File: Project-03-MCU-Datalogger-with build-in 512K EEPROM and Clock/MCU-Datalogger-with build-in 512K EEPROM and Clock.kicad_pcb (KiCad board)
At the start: 2 copper layers, 49.2 x 33.5 mm, 30 parts, among them J1 Conn_01x09_Pin, J2 Conn_01x04_Pin, J4 Conn_02x03_Odd_Even, U1 DS1337S_, U2 24LC1025, U3 24LC1025, U4 ATMEGA328P-AU, Y1 32.768 khz, Y2 16 Mhz

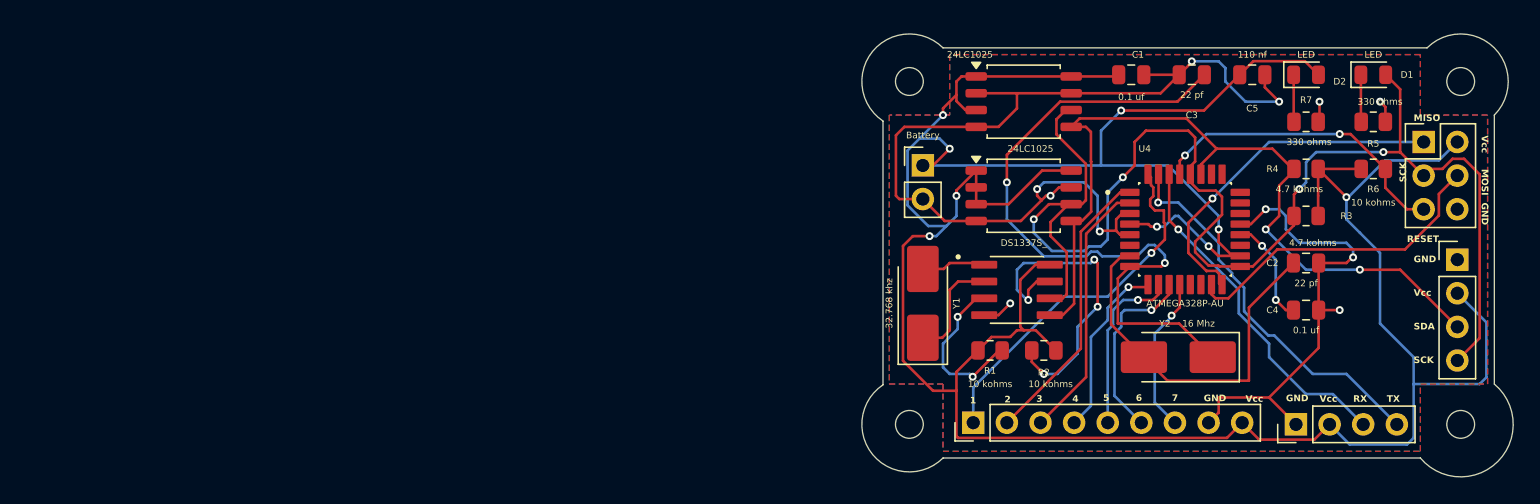
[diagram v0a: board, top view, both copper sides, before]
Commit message: small changes
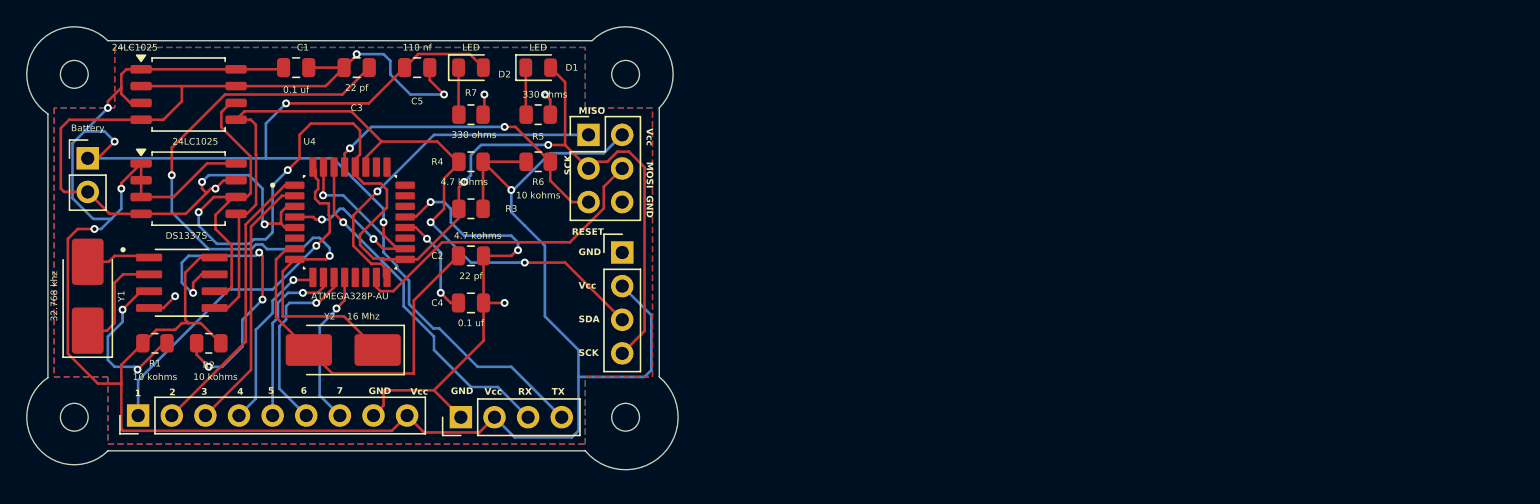
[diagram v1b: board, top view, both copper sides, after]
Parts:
- moved C2 63.1 mm to (85.2, 70.6)
- moved C4 63.1 mm to (85.2, 74.1)
- moved D2 63.1 mm to (85.2, 56.4)
- moved H3 63.1 mm to (96.9, 56.9)
- moved H4 63.1 mm to (96.9, 82.8)
- moved J3 63.1 mm to (84.5, 82.8)
- moved R3 63.1 mm to (85.2, 67.0)
- moved R4 63.1 mm to (85.2, 63.5)
- moved R7 63.1 mm to (85.2, 59.9)
- moved U4 63.1 mm to (76.1, 68.0)
- moved H1 63.1 mm to (55.3, 56.9)
- moved H2 63.1 mm to (55.3, 82.8)
- moved U1 63.1 mm to (63.4, 72.6)
- moved BT1 63.1 mm to (56.3, 63.2)
- moved D1 63.1 mm to (90.3, 56.4)
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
